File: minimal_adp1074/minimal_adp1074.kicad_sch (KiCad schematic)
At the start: 65 parts, among them Q1 80 V, Q2 -60 V, Q3 40 V, Q4 40 V, T1 PL160X9-102L-BLD, U1 ADP1074ACCZ-R7

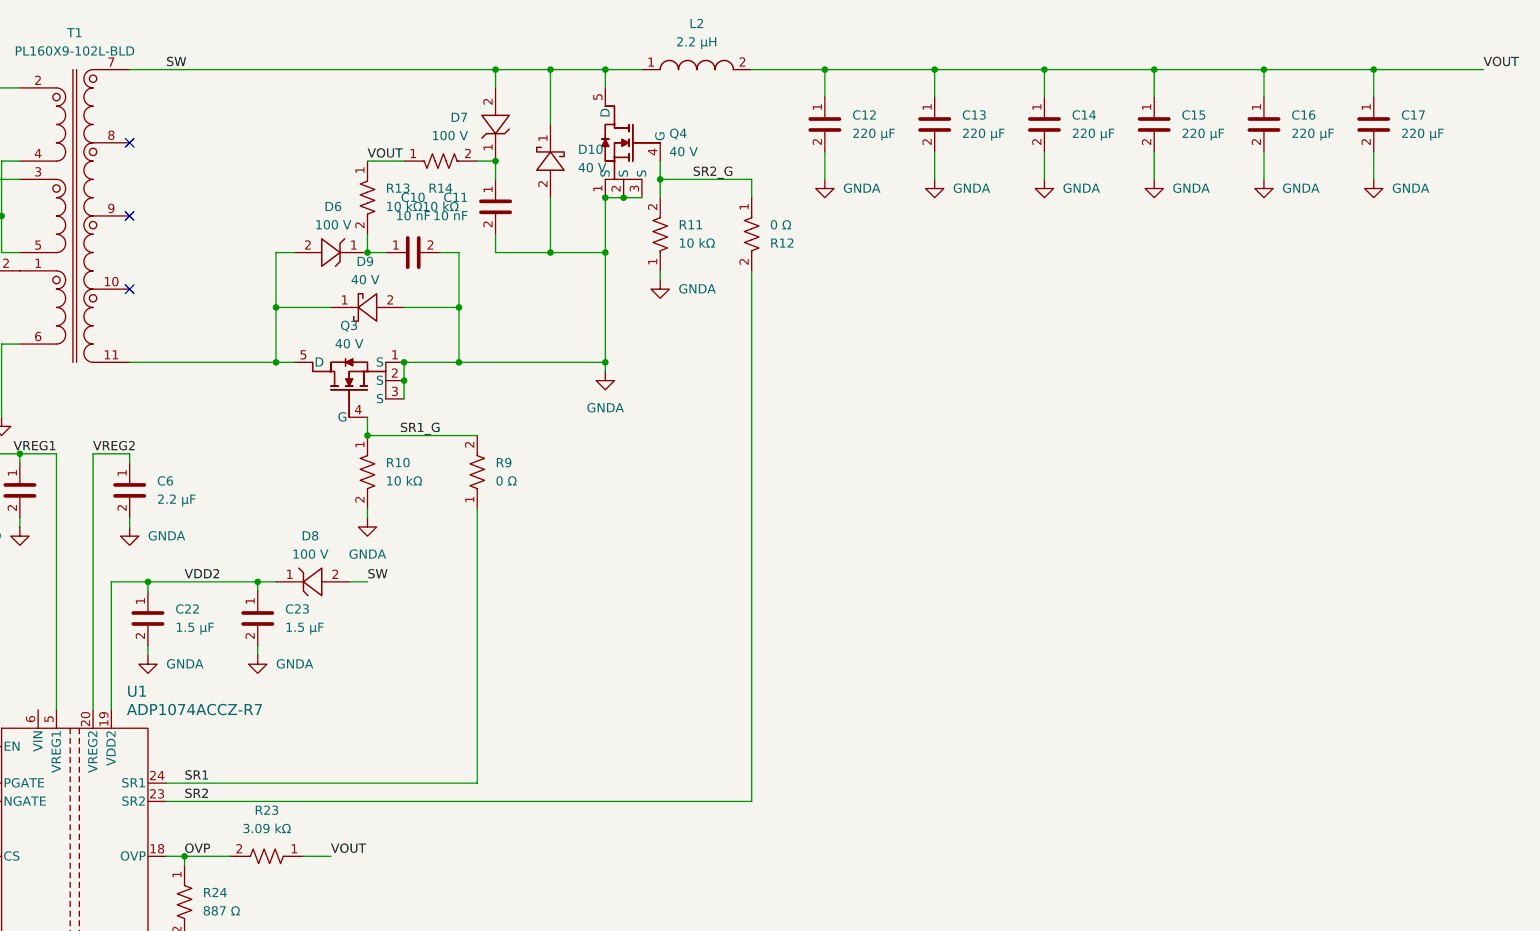
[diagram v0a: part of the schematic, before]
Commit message: backup
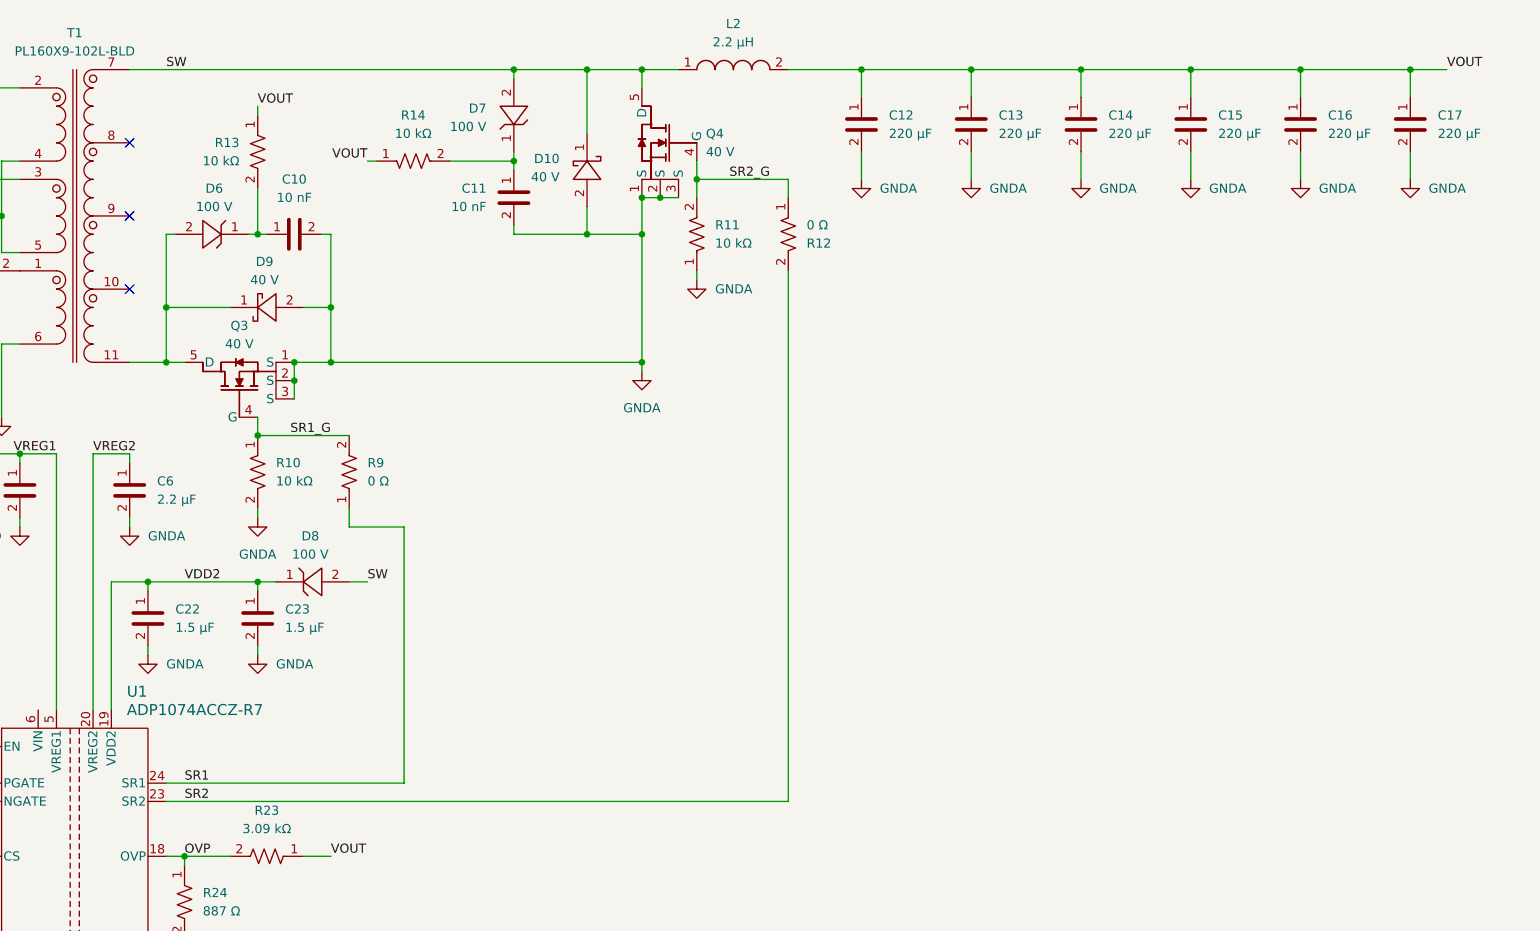
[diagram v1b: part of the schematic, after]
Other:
- moved on the sheet: C10, C11, C12, C13, C14, C15, C16, C17, D10, D6, D7, D9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
